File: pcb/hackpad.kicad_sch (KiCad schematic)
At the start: 33 parts, among them J1 Conn_01x04, J2 Conn_01x04, SW1 SW_Push, SW2 SW_Push, SW3 SW_Push, SW4 SW_Push, SW5 SW_Push, SW6 SW_Push, SW7 SW_Push, SW8 SW_Push, SW9 RotaryEncoder_Switch, U1 MOUDLE-SEEEDUINO-XIAO

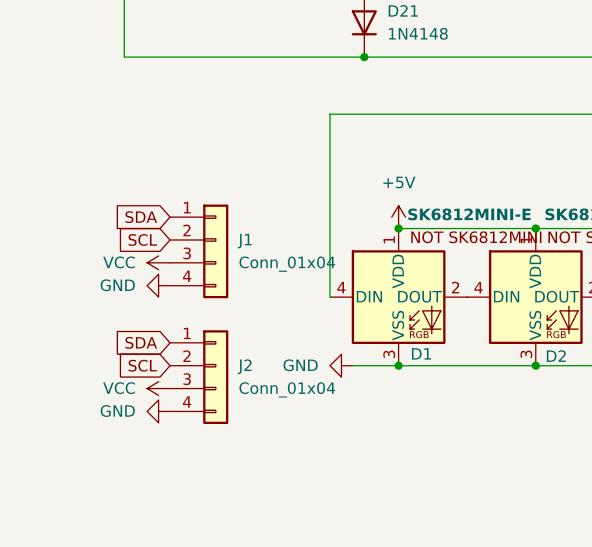
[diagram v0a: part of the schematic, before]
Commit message: v2
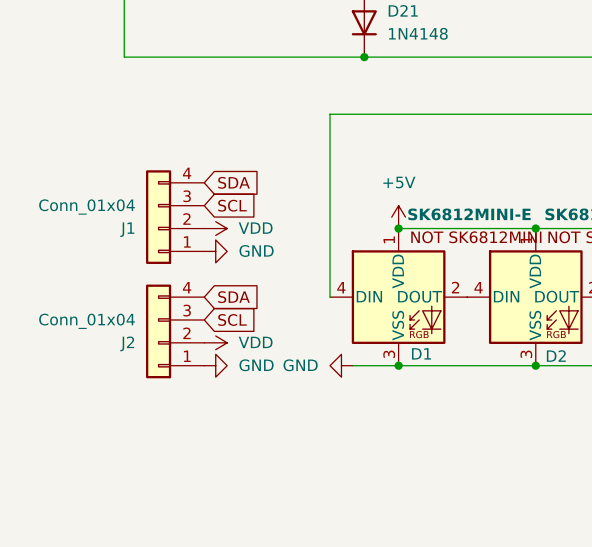
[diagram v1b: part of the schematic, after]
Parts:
- D1, D10, D11, D12, D2, D3, D4, D5, D6, D7, D8, D9: footprint LED_SMD:LED_WS2812B_PLCC4_5.0x5.0mm_P3.2mm -> footprints:SK6812MINI-E_fixed
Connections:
- net VCC is gone; now on net SCL: J1.3 (Pin_3), J2.3 (Pin_3)
- net GND: now also J1.1 (Pin_1), J2.1 (Pin_1); no longer J1.4 (Pin_4), J2.4 (Pin_4)
- net SCL: no longer J1.2 (Pin_2), J2.2 (Pin_2)
- net SDA: now also J1.4 (Pin_4), J2.4 (Pin_4); no longer J1.1 (Pin_1), J2.1 (Pin_1)
- net VDD: now also J1.2 (Pin_2), J2.2 (Pin_2)
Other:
- moved on the sheet: J1, J2
